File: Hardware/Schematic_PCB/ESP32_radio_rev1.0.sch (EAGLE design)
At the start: 35 parts, among them CON1 ENCODER1, CON2 ENCODER2, CON3 OLED Display, CON4 SD Card, CON5 Audio, CON6 JOY / SWITCHES

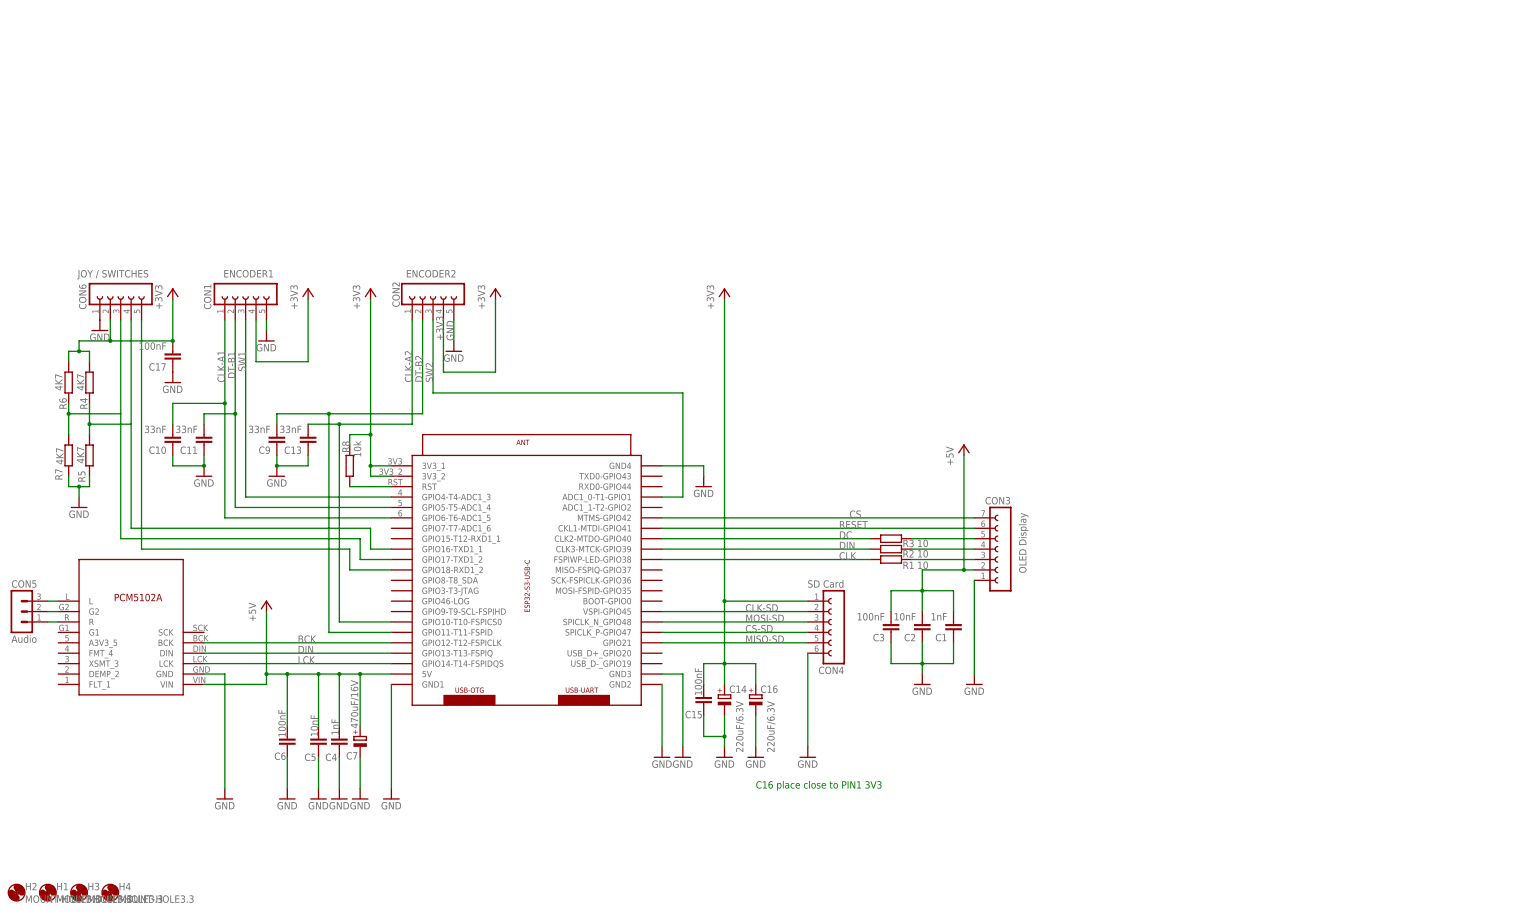
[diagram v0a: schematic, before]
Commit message: Update
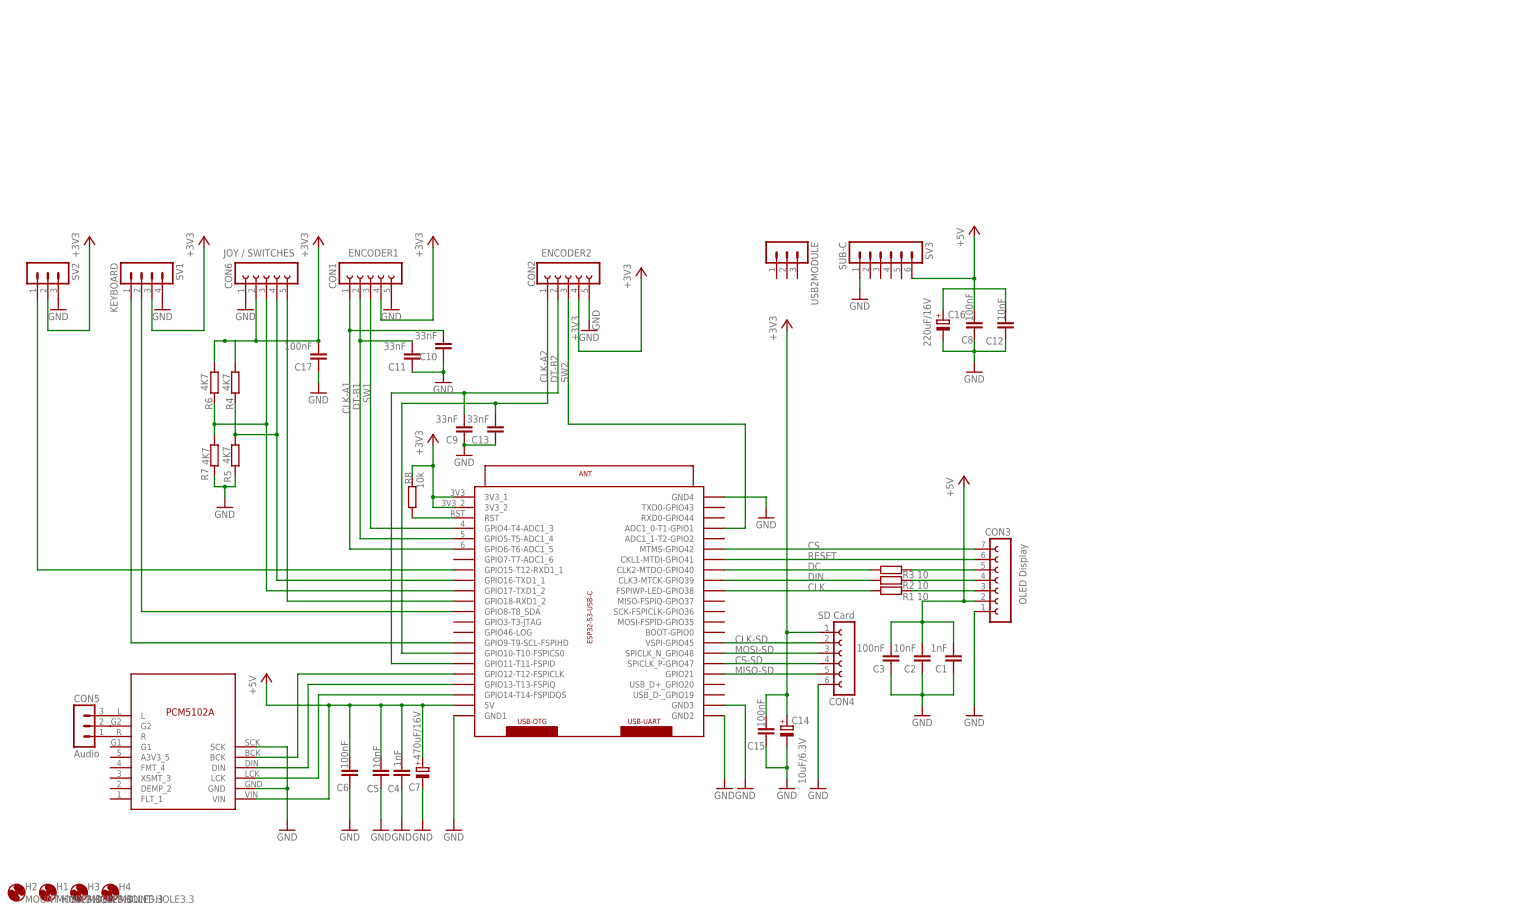
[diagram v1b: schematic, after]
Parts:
- added C12: 10nF, rcl:C-EUC0603
- added C8: 100nF, rcl:C-EUC0603
- added SV1: KEYBOARD, con-lstb:MA04-1
- added SV2, USB2MODULE: (no value), con-lstb:MA03-1
- added SV3: SUB-C, con-lstb:MA06-1
- C14: value 220uF/6.3V -> 10uF/6.3V
- C16: value 220uF/6.3V -> 220uF/16V
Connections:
- net BCK renamed N$15
- net LCK renamed N$10
- new net I2C: SV1.2, U$1.GPIO8-T8_SDA
- new net I2C_ADC: SV1.1, U$1.GPIO9-T9-SCL-FSPIHD
- new net N$14: U$1.GPIO13-T13-FSPIQ, U$2.DIN
- new net N$18: SV2.1, U$1.GPIO15-T12-RXD1_1
- net +3V3: now also SV1.3, SV2.2; no longer C16.+
- net +5V: now also C12.2, C16.+, C8.2, SV3.6
- net DIN: no longer U$1.GPIO13-T13-FSPIQ, U$2.DIN
- net GND: now also C12.1, C8.1, SV1.4, SV2.3, SV3.1, U$2.SCK
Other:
- note removed: "C16 place close to PIN1 3V3"
- moved on the sheet: C1, C10, C11, C13, C14, C15, C16, C17, C2, C3, C4, C5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

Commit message: Schematic & PCB update
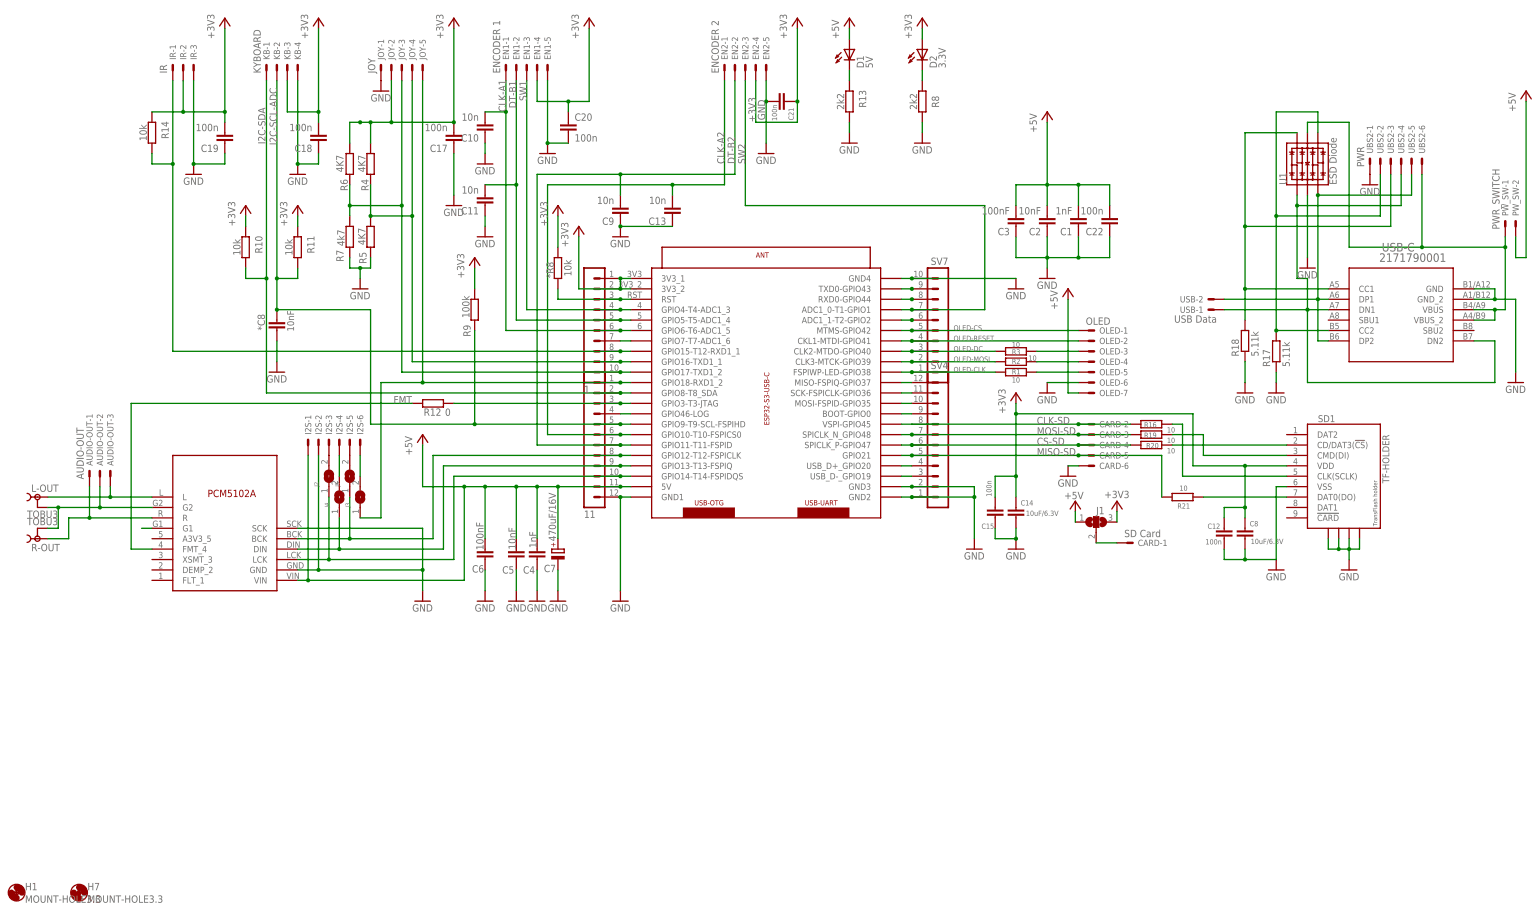
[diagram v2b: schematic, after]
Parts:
- removed C16: 220uF/16V, rcl:CPOL-EU150CLZ-1010
- removed CON1: ENCODER1, con-lsta:FE05-1
- removed CON2: ENCODER2, con-lsta:FE05-1
- removed CON3: OLED Display, con-lsta:FE07-1
- removed CON4: SD Card, con-lsta:FE06-1
- removed CON5: Audio, con-lstb:MA03-1
- removed CON6: JOY / SWITCHES, con-lsta:FE05-1
- removed H2, H4: MOUNT-HOLE3.3, holes:MOUNT-HOLE3.3
- removed SV1: KEYBOARD, con-lstb:MA04-1
- removed SV2, USB2MODULE: (no value), con-lstb:MA03-1
- removed SV3: SUB-C, con-lstb:MA06-1
- removed U$2: I2S_PCM_51XX_SOUNDCARD, PCM5102A:I2S_PCM_51XX_SOUNDCARD
- added *C8: 10nF, rcl:C-EUC0603
- added *R8, R10, R11, R14: 10k, rcl:R-EU_R0603
- added 1: (no value), con-goldpins:MA10-1
- added 11, SV4: (no value), con-goldpins:MA12-1
- added AUDIO-OUT: AUDIO-OUT, JST XH Connectors v1-0:JST-XH-03-PIN-LONG-PAD
- added C18, C19, C20, C21, C22: 100n, rcl:C-EUC0603
- added CARD: SD Card, JST XH Connectors v1-0:JST-XH-06-PIN-LONG-PAD
- added D1: 5V, led:LEDCHIP-LED0805
- added D2: 3.3V, led:LEDCHIP-LED0805
- added EN1: ENCODER 1, JST XH Connectors v1-0:JST-XH-05-PIN-LONG-PAD
- added EN2: ENCODER 2, JST XH Connectors v1-0:JST-XH-05-PIN-LONG-PAD
- added I2S: JST-XH-06-PIN-LONG-PAD, JST XH Connectors v1-0:JST-XH-06-PIN-LONG-PAD
- added IR: IR, JST XH Connectors v1-0:JST-XH-03-PIN-LONG-PAD
- added J1: (no value), jumper:SJ2W
- added J2, J3, J4, J5: (no value), jumper:SJ
- added JOY: JOY, JST XH Connectors v1-0:JST-XH-05-PIN-LONG-PAD
- added KB: KYBOARD, JST XH Connectors v1-0:JST-XH-04-PIN-LONG-PAD
- added L-OUT, R-OUT: TOBU3, con-hirschmann:TOBU3
- added M2: I2S_PCM_51XX_SOUNDCARD, PCM5102A:I2S_PCM_51XX_SOUNDCARD
- added OLED: OLED, JST XH Connectors v1-0:JST-XH-07-PIN-LONG-PAD
- added PW_SW: PWR_SWITCH, JST XH Connectors v1-0:JST-XH-02-PIN-LONG-PAD
- added R12: 0, rcl:R-EU_R0603
- added R13: 2k2, rcl:R-EU_R0603
- added R16, R19, R20, R21: 10, rcl:R-EU_R0603
- added R17, R18: 5.11k, rcl:R-EU_R0603
- added R9: 100k, rcl:R-EU_R0603
- added SD1: TF-HOLDER, sd-mmc:TF-HOLDER
- added SV7: (no value), con-lstb:MA10-1
- added U1: ESD Diode, SparkFun-DiscreteSemi:TVS_DIODE_ARRAY_DT1042-04SO-7
- added UBS2: PWR, JST XH Connectors v1-0:JST-XH-06-PIN-LONG-PAD
- added USB: USB Data, JST XH Connectors v1-0:JST-XH-02-PIN-LONG-PAD
- added USB-C: 2171790001, USB-C_2:2171790001
- C10, C11, C13, C9: value 33nF -> 10n
- C12: value 10nF -> 100n
- C14: device rcl:CPOL-EU150CLZ-1010 -> rcl:C-EUC1210
- C15, C17: value 100nF -> 100n
- C8: value 100nF -> 10uF/6.3V; device rcl:C-EUC0603 -> rcl:C-EUC1210
- R7: value 4K7 -> 4k7
- R8: value 10k -> 2k2
- renumbered H3 to H7
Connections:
- removed net CLK: R1.1, U$1.FSPIWP-LED-GPIO38
- removed net CS: CON3.7, U$1.MTMS-GPIO42
- removed net DC: R3.1, U$1.CLK2-MTDO-GPIO40
- removed net DIN: R2.1, U$1.CLK3-MTCK-GPIO39
- removed net I2C: SV1.2, U$1.GPIO8-T8_SDA
- removed net I2C_ADC: SV1.1, U$1.GPIO9-T9-SCL-FSPIHD
- removed net RESET: CON3.6, U$1.CKL1-MTDI-GPIO41
- new net 5V_USB: PW_SW-1.S, U1.VCC, UBS2-6.S, USB-C.VBUS, USB-C.VBUS_2
- new net ANALOGGND: AUDIO-OUT-2.S, L-OUT.2, M2.G2, R-OUT.2
- new net FMT: M2.FMT_4, R12.2
- new net FMT1: 11.4, U$1.GPIO46-LOG
- new net I2C-SCL-ADC: *C8.1, 11.5, KB-2.S, R11.1, R9.1, U$1.GPIO9-T9-SCL-FSPIHD
- new net I2C-SDA: 11.2, KB-1.S, R10.1, U$1.GPIO8-T8_SDA
- new net N$12: R20.2, SD1.CD/DAT3(!CS!)
- new net N$16: 1.7, U$1.GPIO7-T7-ADC1_6
- new net N$17: SV7.6, U$1.ADC1_1-T2-GPIO2
- new net N$19: D2.C, R8.2
- new net N$20: SV7.8, U$1.RXD0-GPIO44
- new net N$21: SV7.9, U$1.TXD0-GPIO43
- new net N$22: SV4.3, U$1.USB_D-_GPIO19
- new net N$23: SV4.4, U$1.USB_D+_GPIO20
- new net N$24: SV4.9, U$1.BOOT-GPIO0
- new net N$25: SV4.10, U$1.MOSI-FSPID-GPIO35
- new net N$26: SV4.11, U$1.SCK-FSPICLK-GPIO36
- new net N$27: SV4.12, U$1.MISO-FSPIQ-GPIO37
- new net N$28: 11.3, R12.1, U$1.GPIO3-T3-JTAG
- new net N$30: D1.C, R13.2
- new net N$31: CARD-1.S, J1.2
- new net N$32: R19.2, SD1.CMD(DI)
- new net N$33: R16.2, SD1.CLK(SCLK)
- new net N$34: U1.IO2, UBS2-5.S, USB-2.S, USB-C.DP1, USB-C.DP2
- new net N$35: U1.IO1, UBS2-4.S, USB-1.S, USB-C.DN1, USB-C.DN2
- new net N$36: I2S-3.S, J2.2
- new net N$37: R17.2, U1.IO3, UBS2-2.S, USB-C.CC2
- new net N$38: R18.2, U1.IO4, UBS2-3.S, USB-C.CC1
- new net N$39: I2S-6.S, J3.2
- new net N$4: OLED-5.S, R1.2
- new net N$40: I2S-5.S, J5.2
- new net N$41: I2S-4.S, J4.2
- new net OLED-CLK: R1.1, SV7.1, U$1.FSPIWP-LED-GPIO38
- new net OLED-CS: OLED-1.S, SV7.5, U$1.MTMS-GPIO42
- new net OLED-DC: R3.1, SV7.3, U$1.CLK2-MTDO-GPIO40
- new net OLED-MOSI: R2.1, SV7.2, U$1.CLK3-MTCK-GPIO39
- new net OLED-RESET: OLED-2.S, SV7.4, U$1.CKL1-MTDI-GPIO41
- net +3V3: now also *R8.1, 1.1, 1.2, C12.2, C14.1, C18.2, C19.2, C20.1, C21.1, C8.1, D2.A, EN1-4.S, EN2-4.S, IR-2.S, J1.3, JOY-2.S, KB-3.S, R10.2, R11.2, R14.2, R9.2, SD1.VDD; no longer C14.+, CON1.4, CON2.4, CON4.1, CON6.2, R8.1, SV1.3, SV2.2
- net +5V: now also 11.11, C22.2, D1.A, I2S-1.S, J1.1, M2.VIN, OLED-7.S, PW_SW-2.S; no longer C12.2, C16.+, C8.2, CON3.2, SV3.6, U$2.VIN
- net CLK-A1: now also 1.6, EN1-1.S; no longer CON1.1
- net CLK-A2: now also 11.6, EN2-1.S; no longer CON2.1
- net CLK-SD: now also CARD-2.S, R16.1, SV4.8; no longer CON4.2
- net CS-SD: now also CARD-4.S, R20.1, SV4.6; no longer CON4.4
- net DT-B1: now also 1.5, EN1-2.S; no longer CON1.2
- net DT-B2: now also 11.7, EN2-2.S; no longer CON2.2
- net GND: now also *C8.2, 11.12, C14.2, C18.1, C19.1, C20.2, C21.2, C22.1, C8.2, CARD-6.S, EN1-5.S, EN2-5.S, I2S-2.S, IR-3.S, JOY-1.S, KB-4.S, M2.GND, M2.SCK, OLED-6.S, R13.1, R17.1, R18.1, R8.1, SD1.S1, SD1.S2, SD1.S3, SD1.S4, SD1.VSS, SV4.1, SV4.2, SV7.10, U1.VSS, UBS2-1.S, USB-C.GND, USB-C.GND_2; no longer C14.-, C16.-, C8.1, CON1.5, CON2.5, CON3.1, CON4.6, CON6.1, SV1.4, SV2.3, SV3.1, U$2.GND, U$2.SCK
- net MISO-SD: now also CARD-5.S, R21.1, SV4.5; no longer CON4.5
- net MOSI-SD: now also CARD-3.S, R19.1, SV4.7; no longer CON4.3
- net N$1: now also AUDIO-OUT-1.S, M2.R, R-OUT.1; no longer CON5.1, U$2.R
- net N$10: now also 11.10, J2.1, M2.LCK; no longer U$2.LCK
- net N$11: now also *R8.2, 1.3; no longer R8.2
- net N$13: now also 1.9, JOY-4.S; no longer CON6.4
- net N$14: now also 11.9, J4.1, M2.DIN; no longer U$2.DIN
- net N$15: now also 11.8, J5.1, M2.BCK; no longer U$2.BCK
- net N$18: now also 1.8, IR-1.S, R14.1; no longer SV2.1
- net N$2: now also M2.G1; no longer CON5.2, U$2.G2
- net N$3: now also AUDIO-OUT-3.S, L-OUT.1, M2.L; no longer CON5.3, U$2.L
- net N$5: now also OLED-4.S, R2.2; no longer CON3.3, R1.2
- net N$6: now also OLED-3.S; no longer CON3.5
- net N$7: now also R21.2, SD1.DAT0(DO); no longer CON3.4, R2.2
- net N$8: now also 1.10, JOY-3.S; no longer CON6.3
- net N$9: now also 11.1, J3.1, JOY-5.S; no longer CON6.5
- net SW1: now also 1.4, EN1-3.S; no longer CON1.3
- net SW2: now also EN2-3.S, SV7.7; no longer CON2.3
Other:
- moved on the sheet: C1, C10, C11, C12, C13, C15, C17, C2, C3, C4, C5, C6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
